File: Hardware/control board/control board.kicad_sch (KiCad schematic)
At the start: 11 parts, among them J1 Screw_Terminal_01x02, SW1 SW_Push

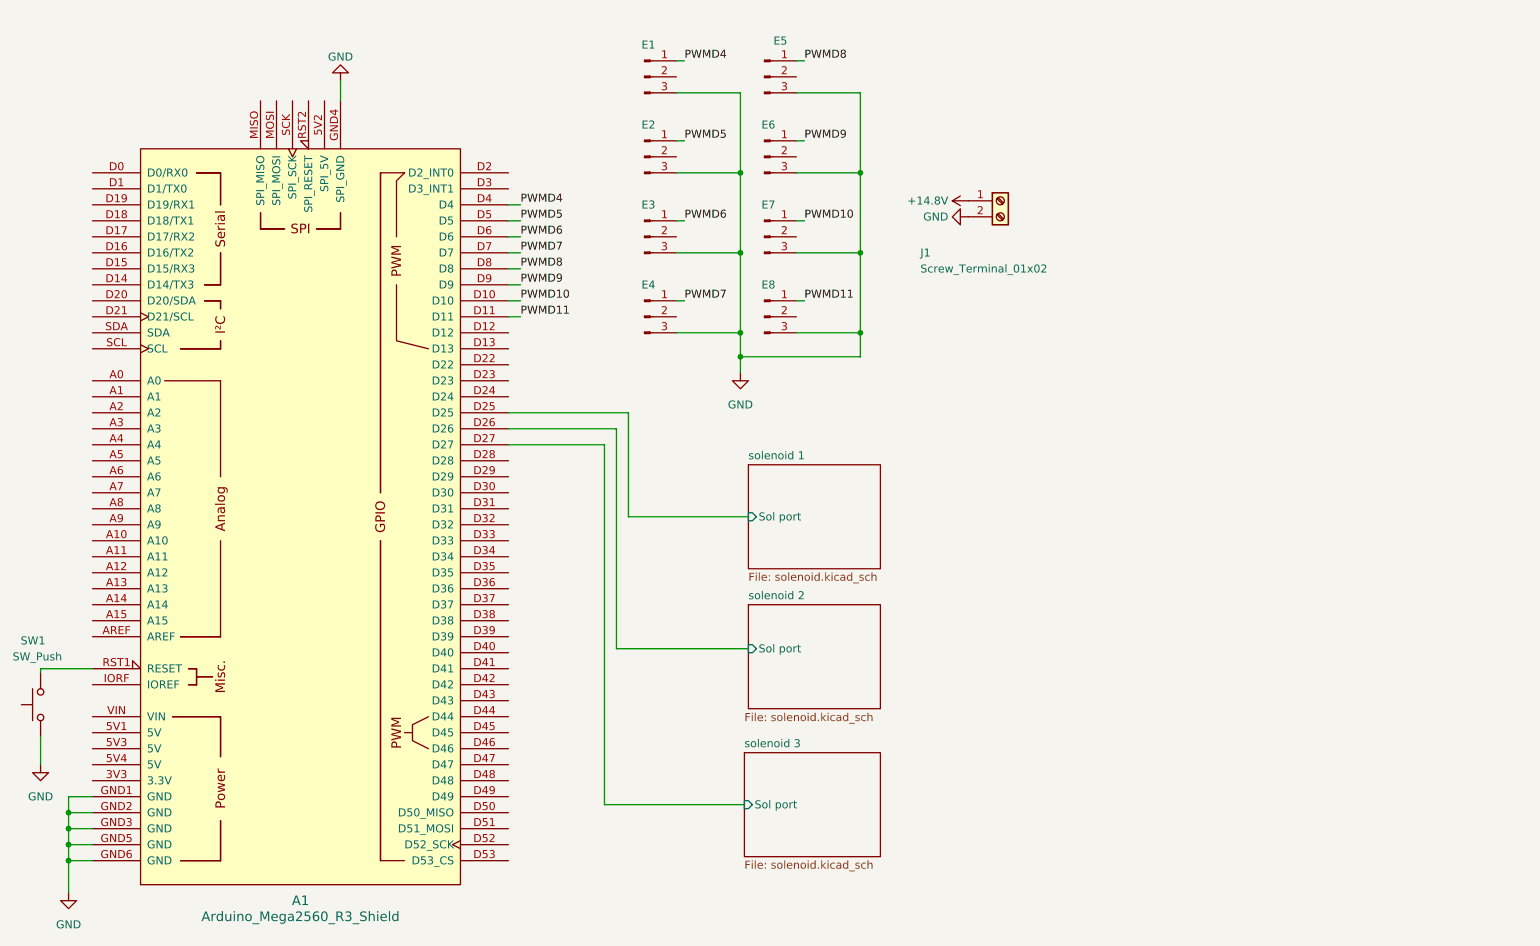
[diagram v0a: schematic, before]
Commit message: schematic formatted
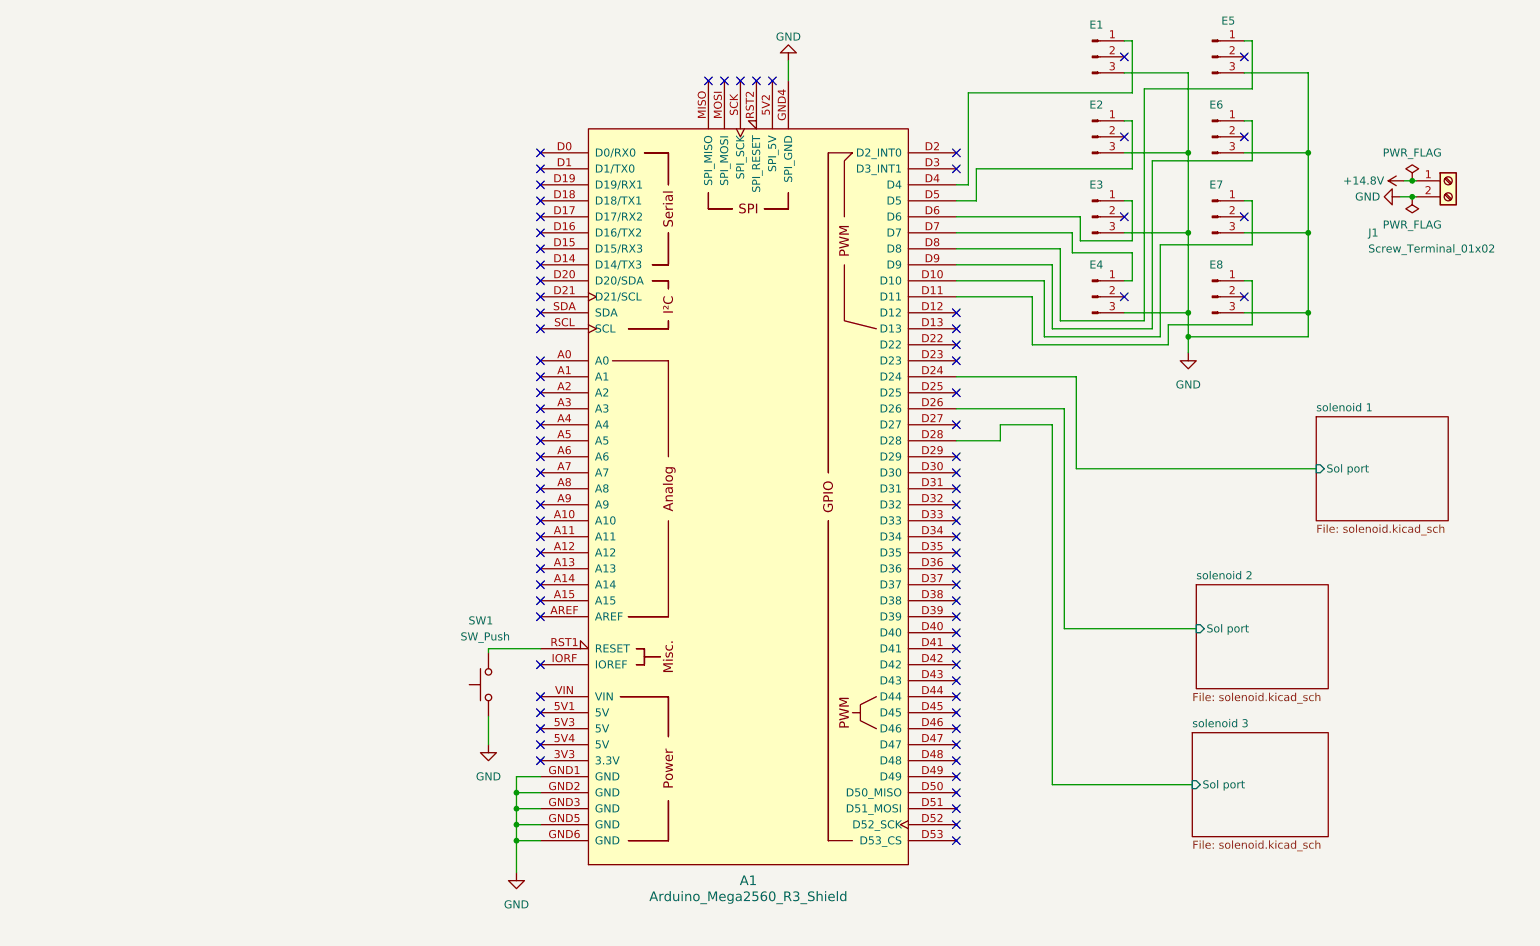
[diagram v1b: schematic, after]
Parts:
- E1, E2, E3, E4, E5, E6, E7, E8: footprint (none) -> Connector_PinHeader_2.54mm:PinHeader_1x03_P2.54mm_Vertical
- J1: footprint (none) -> TerminalBlock_Phoenix:TerminalBlock_Phoenix_MPT-0,5-2-2.54_1x02_P2.54mm_Horizontal
- SW1: footprint (none) -> Button_Switch_THT:SW_PUSH_6mm
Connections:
- net solenoid 1/Sol port: now also A1.D24; no longer A1.D25
- net solenoid 3/Sol port: now also A1.D28; no longer A1.D27
- net PWMD10: no longer names the net of A1.D10, E7.1 (Pin_1)
- net PWMD11: no longer names the net of A1.D11, E8.1 (Pin_1)
- net PWMD4: no longer names the net of A1.D4, E1.1 (Pin_1)
- net PWMD5: no longer names the net of A1.D5, E2.1 (Pin_1)
- net PWMD6: no longer names the net of A1.D6, E3.1 (Pin_1)
- net PWMD7: no longer names the net of A1.D7, E4.1 (Pin_1)
- net PWMD8: no longer names the net of A1.D8, E5.1 (Pin_1)
- net PWMD9: no longer names the net of A1.D9, E6.1 (Pin_1)
- no-connect marks 0 -> 81
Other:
- moved on the sheet: A1, E1, E2, E3, E4, E5, E6, E7, E8, J1, SW1

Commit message: Revert "Merge branch 'hardware' of https://github.com/bruin-underwater-robotics/2023-2024 into hardware"
This reverts commit f5050c74fbd2d727488e15b71bfb24c9149407df, reversing
changes made to d4ffa11f2369dfdbeb25d57bd1642de1ab50c466.
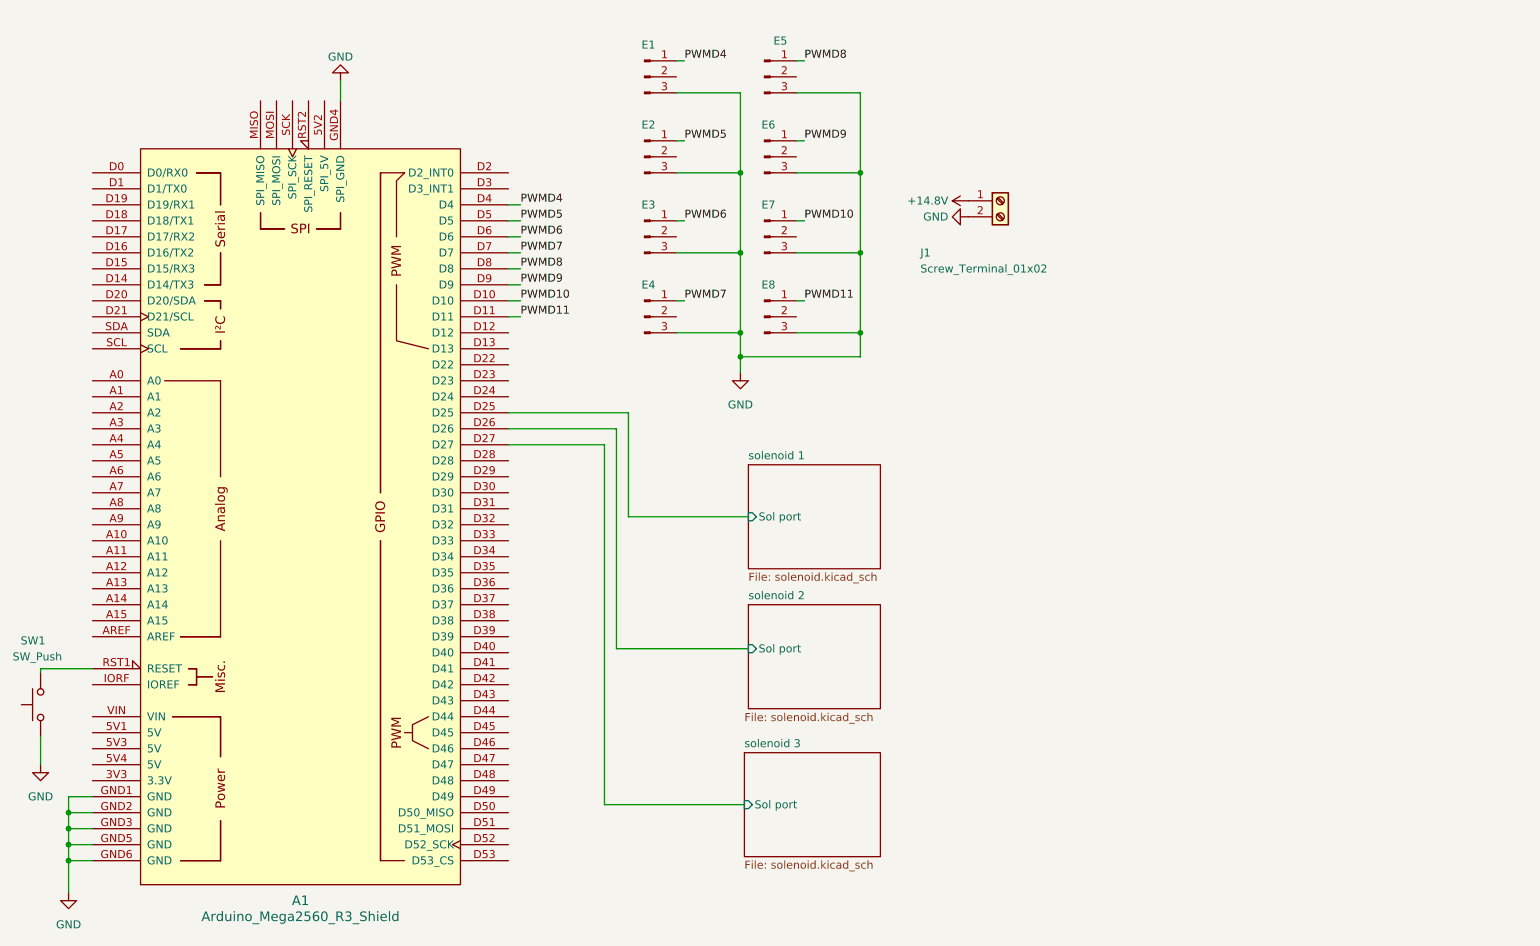
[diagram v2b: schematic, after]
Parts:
- E1, E2, E3, E4, E5, E6, E7, E8: footprint Connector_PinHeader_2.54mm:PinHeader_1x03_P2.54mm_Vertical -> (none)
- J1: footprint TerminalBlock_Phoenix:TerminalBlock_Phoenix_MPT-0,5-2-2.54_1x02_P2.54mm_Horizontal -> (none)
- SW1: footprint Button_Switch_THT:SW_PUSH_6mm -> (none)
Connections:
- net solenoid 1/Sol port: now also A1.D25; no longer A1.D24
- net solenoid 3/Sol port: now also A1.D27; no longer A1.D28
- net PWMD10: now reaches A1.D10, E7.1 (Pin_1)
- net PWMD11: now reaches A1.D11, E8.1 (Pin_1)
- net PWMD4: now reaches A1.D4, E1.1 (Pin_1)
- net PWMD5: now reaches A1.D5, E2.1 (Pin_1)
- net PWMD6: now reaches A1.D6, E3.1 (Pin_1)
- net PWMD7: now reaches A1.D7, E4.1 (Pin_1)
- net PWMD8: now reaches A1.D8, E5.1 (Pin_1)
- net PWMD9: now reaches A1.D9, E6.1 (Pin_1)
- no-connect marks 81 -> 0
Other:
- moved on the sheet: A1, E1, E2, E3, E4, E5, E6, E7, E8, J1, SW1
